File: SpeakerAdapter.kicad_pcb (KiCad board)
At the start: 2 copper layers, 2 parts, among them J1 Terminal Block, J2 JST-PH

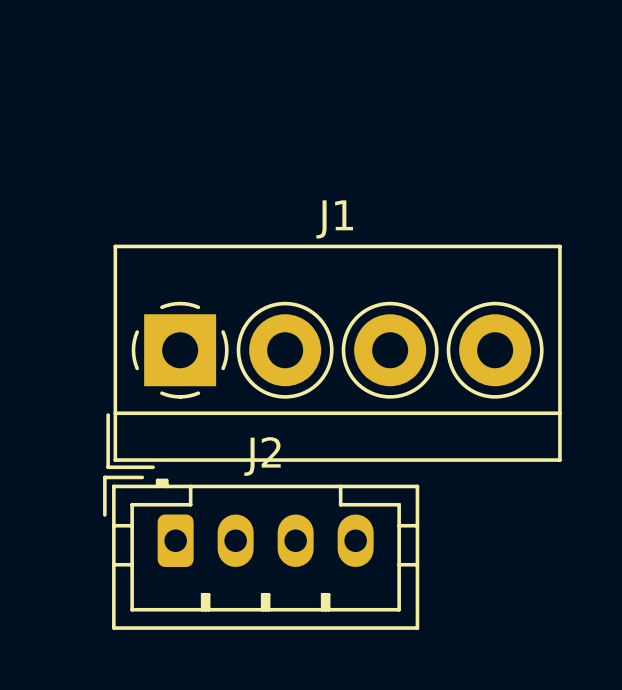
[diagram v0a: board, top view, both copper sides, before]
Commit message: Position footprints.
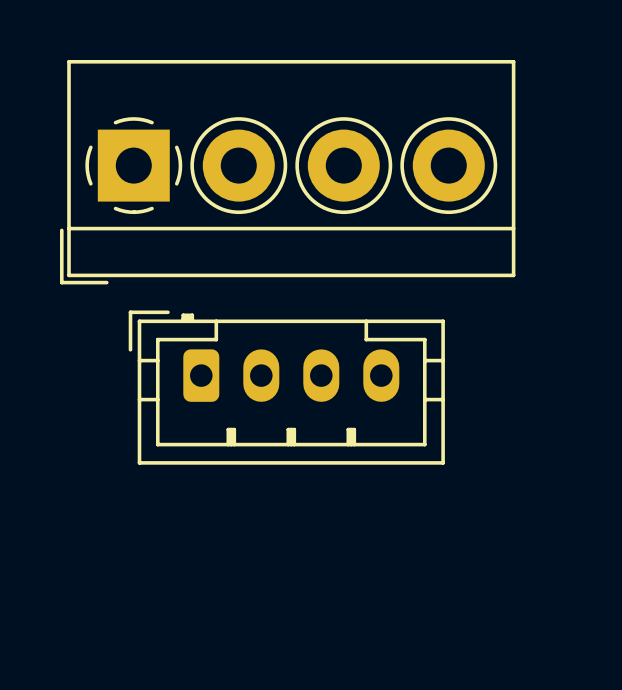
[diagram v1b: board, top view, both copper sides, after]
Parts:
- moved J1 6.35 mm to (154.8, 60.0)
- moved J2 5.57 mm to (157.0, 67.0)
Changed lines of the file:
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@@
     (47 F.CrtYd user)
     (48 B.Fab user)
-    (49 F.Fab user)
+    (49 F.Fab user hide)
   )
   (setup
@@
   )
   (module TerminalBlock_4Ucon:TerminalBlock_4Ucon_1x04_P3.50mm_Horizontal (layer F.Cu)
-    (at 156.295001 66.155001)
+    (at 154.75 60)
     (descr "Terminal Block 4Ucon ItemNo. 20001, 4 pins, pitch 3.5mm, size 14.7x7mm^2, drill diamater 1.2mm, pad diameter 2.4mm, see http://www.4uconnector.com/online/object/4udrawing/20001.pdf, script-generated using https://github.com/pointhi/kicad-footprint-generator/scripts/TerminalBlock_4Ucon")
     (tags "THT Terminal Block 4Ucon ItemNo. 20001 pitch 3.5mm size 14.7x7mm^2 drill 1.2mm pad 2.4mm")
-    (fp_text reference J1 (at 5.25 -4.46) (layer F.SilkS)
+    (fp_text reference J1 (at 5.25 -4.46) (layer F.SilkS) hide
       (effects (font (size 1 1) (thickness 0.15)))
     )
@@
   )
   (module Connector_JST:JST_PH_B4B-PH-K_1x04_P2.00mm_Vertical (layer F.Cu)
-    (at 156.145001 72.505001)
+    (at 157 67)
     (descr "JST PH series connector, B4B-PH-K (http://www.jst-mfg.com/product/pdf/eng/ePH.pdf), generated with kicad-footprint-generator")
     (tags "connector JST PH side entry")
-    (fp_text reference J2 (at 3 -2.9) (layer F.SilkS)
+    (fp_text reference J2 (at 3 -2.9) (layer F.SilkS) hide
       (effects (font (size 1 1) (thickness 0.15)))
     )
